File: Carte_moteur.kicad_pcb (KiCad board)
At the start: 2 copper layers, 117 parts, among them J101 Conn_01x02_Socket, J102 Conn_01x02, J103 Conn_01x02, J104 Conn_01x07, J201 Conn_01x05_Pin, J202 Conn_01x04_Pin, J301 Conn_01x05_Pin, J302 Conn_01x04_Pin, J401 Conn_01x05_Pin, J402 Conn_01x04_Pin, J601 Conn_01x06_Pin, J602 USB_B_Mini, Q601 MMBTA44, SW301 SW_DIP_x02, SW302 SW_DIP_x02, SW303 SW_DIP_x02, U101 LD1117S33TR_SOT223, U201 TMC2209, U301 TMC2209, U401 TMC2209, U501 STM32G474RETx, U601 ECMF02-2AMX6, U602 LD1117S33TR_SOT223, U603 STM32F103CBTx, Y601 Crystal_GND24

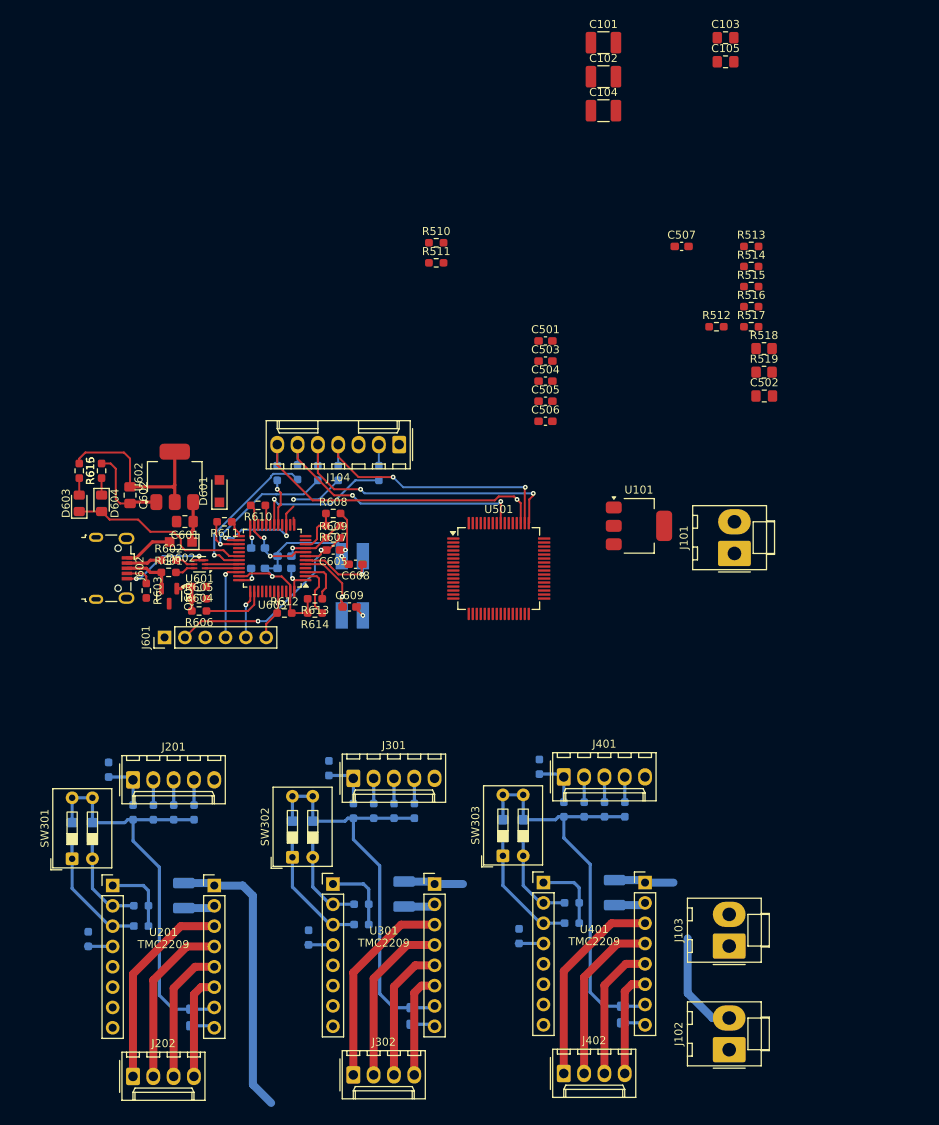
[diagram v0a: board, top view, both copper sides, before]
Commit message: hrtim
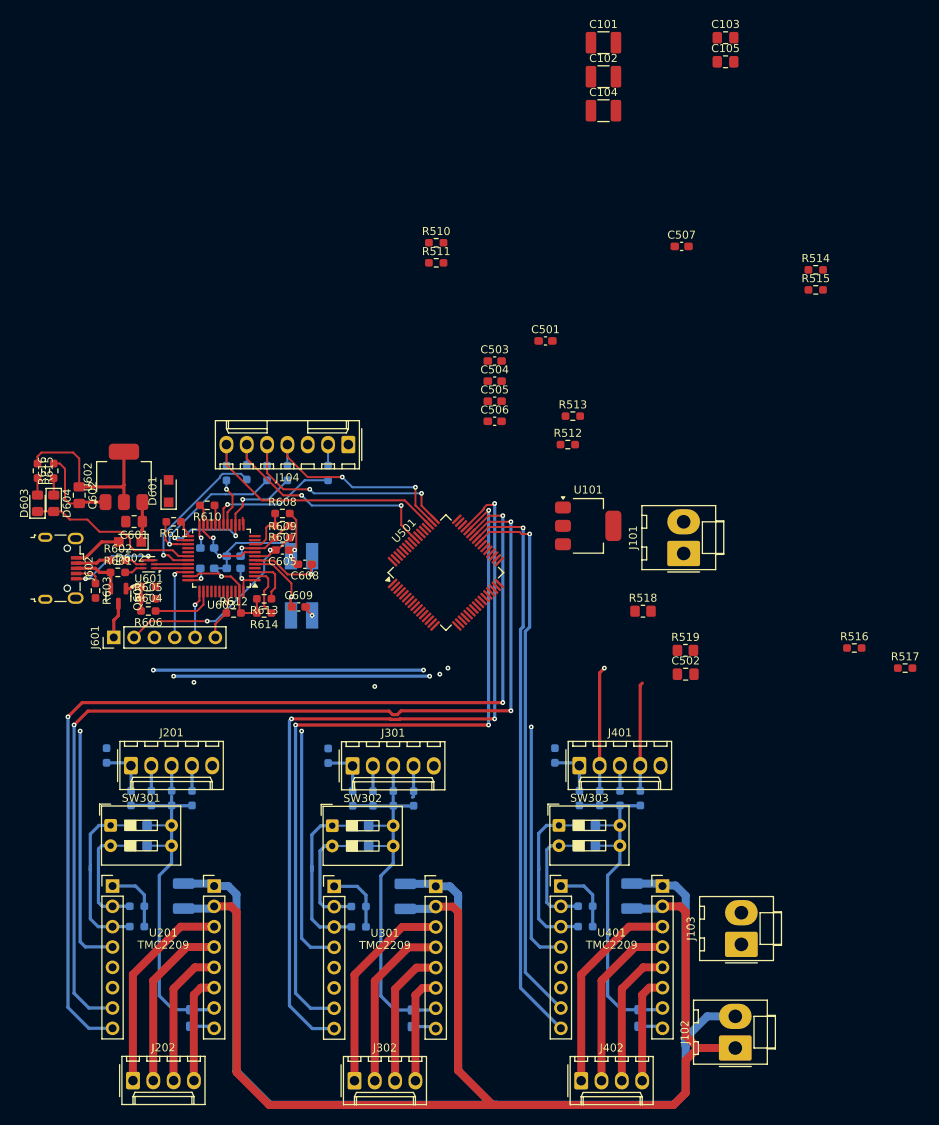
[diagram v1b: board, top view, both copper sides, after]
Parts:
- removed R205, R305, R405: R_US, Resistor_SMD:R_0603_1608Metric_Pad0.98x0.95mm_HandSolder
- moved R517 46.8 mm to (186.9, 117.1)
- moved R516 44.6 mm to (180.6, 114.6)
- moved R518 36.1 mm to (154.2, 110.0)
- moved C502 36.1 mm to (159.5, 117.9)
- moved R519 36.1 mm to (159.5, 114.9)
- moved R513 30.8 mm to (145.4, 85.6)
- moved R512 23.7 mm to (144.8, 89.2)
- moved R406 10.6 mm to (147.2, 136.8), turned to 180 degrees
- moved R306 8.55 mm to (118.9, 136.8), turned to 180 degrees
- moved R206 8.41 mm to (91.2, 136.8), turned to 180 degrees
- moved R403 8.34 mm to (147.2, 139.3), turned to 180 degrees
- moved R514 8.07 mm to (175.8, 67.3)
- moved R515 8.07 mm to (175.8, 69.8)
- moved SW303 7.97 mm to (143.7, 136.8), turned to 0 degrees
- moved U501 6.62 mm to (129.5, 105.2), turned to 45 degrees
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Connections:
- U201 pad 4: Net-(R205-Pad2) -> /micro/TMC1
- U301 pad 4: Net-(R305-Pad2) -> /micro/TMC2
- U401 pad 4: Net-(R405-Pad2) -> /micro/TMC3
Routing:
- net GND: track 120.7 -> 260.7 mm
- net /micro/HRTIM_CHA2: track 0.00 -> 126.3 mm, vias 0 -> 3
- net /micro/HRTIM_CHA1: track 0.00 -> 123.8 mm, vias 0 -> 3
- net +BATT: track 63.2 -> 164.4 mm
- net /micro/HRTIM_CHB2: track 0.00 -> 100.1 mm, vias 0 -> 3
- net /micro/HRTIM_CHB1: track 0.00 -> 93.7 mm, vias 0 -> 3
- net /micro/HRTIM_CHE2: track 0.00 -> 71.3 mm, vias 0 -> 1
- net /micro/HRTIM_CHE1: track 0.00 -> 68.2 mm, vias 0 -> 1
- net /micro/TIM1_CH1: track 3.16 -> 36.9 mm, vias 0 -> 2
- net /micro/TIM1_CH2: track 3.16 -> 35.2 mm, vias 0 -> 2
- net /micro/TMC3: track 0.00 -> 30.6 mm, vias 0 -> 1
- net /micro/TMC2: track 0.00 -> 30.4 mm, vias 0 -> 1
- net /micro/TMC1: track 0.00 -> 30.3 mm, vias 0 -> 1
- net +3V3: track 156.9 -> 139.0 mm, vias 0 -> 1
- net /micro/TIM5_CH1: track 3.16 -> 15.6 mm, vias 0 -> 2
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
